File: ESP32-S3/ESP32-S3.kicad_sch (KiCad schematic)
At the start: 4 parts, among them J1 Conn_01x08, J2 FlySky Receiver, J3 Conn_01x08, U1 ESP32-S3-DevKitC-1-N32R16V

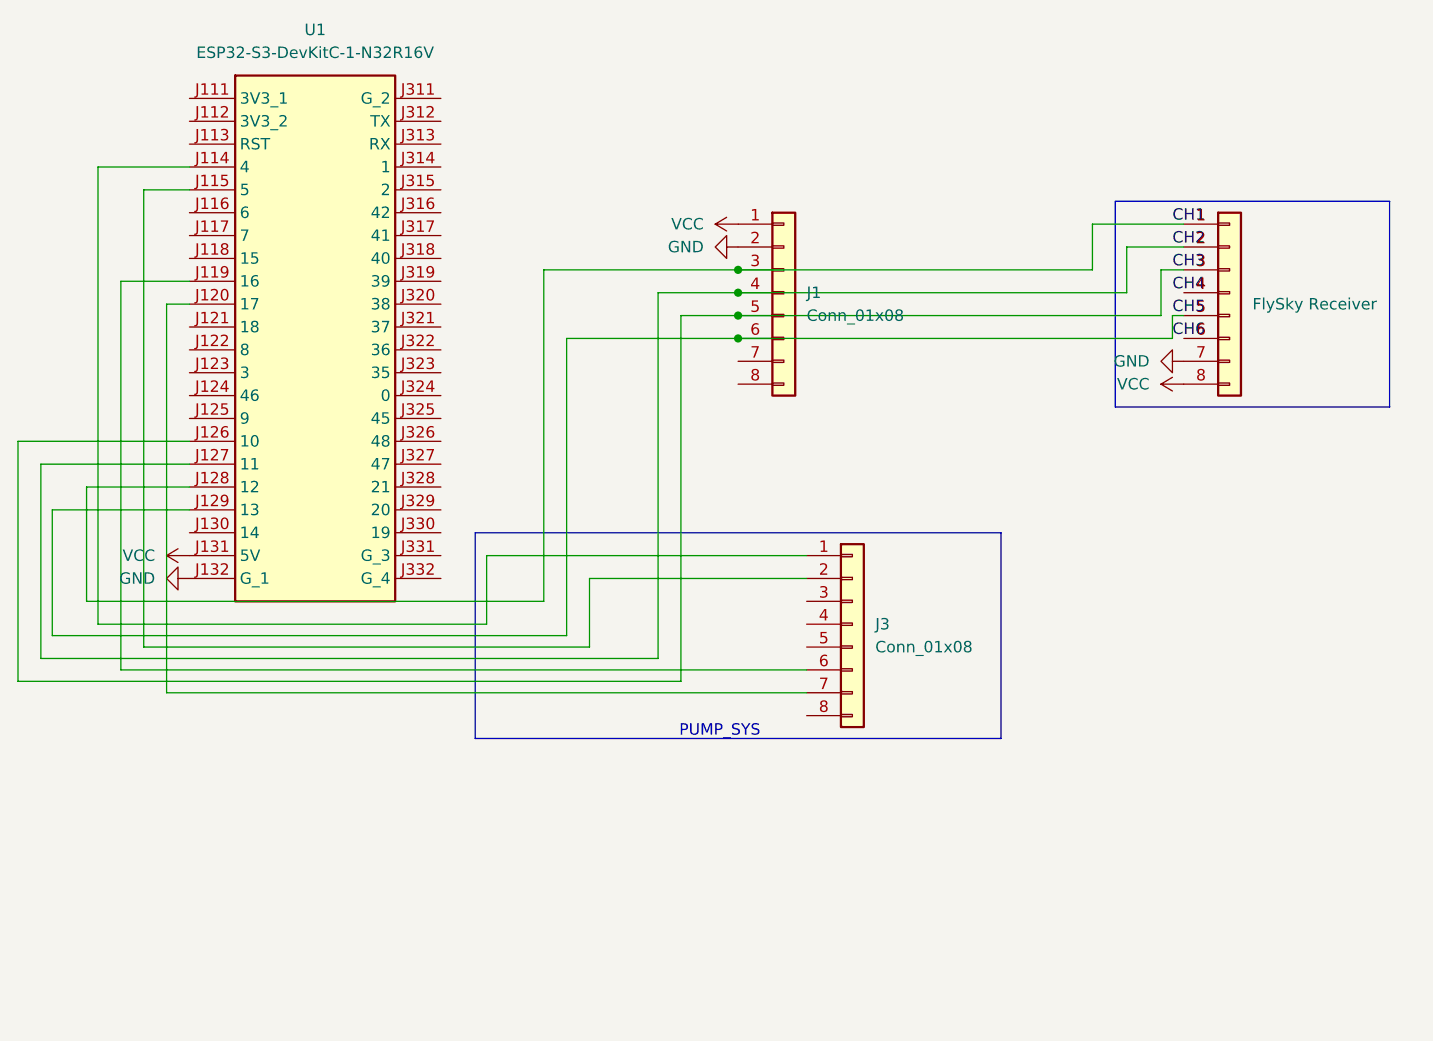
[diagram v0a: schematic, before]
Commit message: Add files via upload
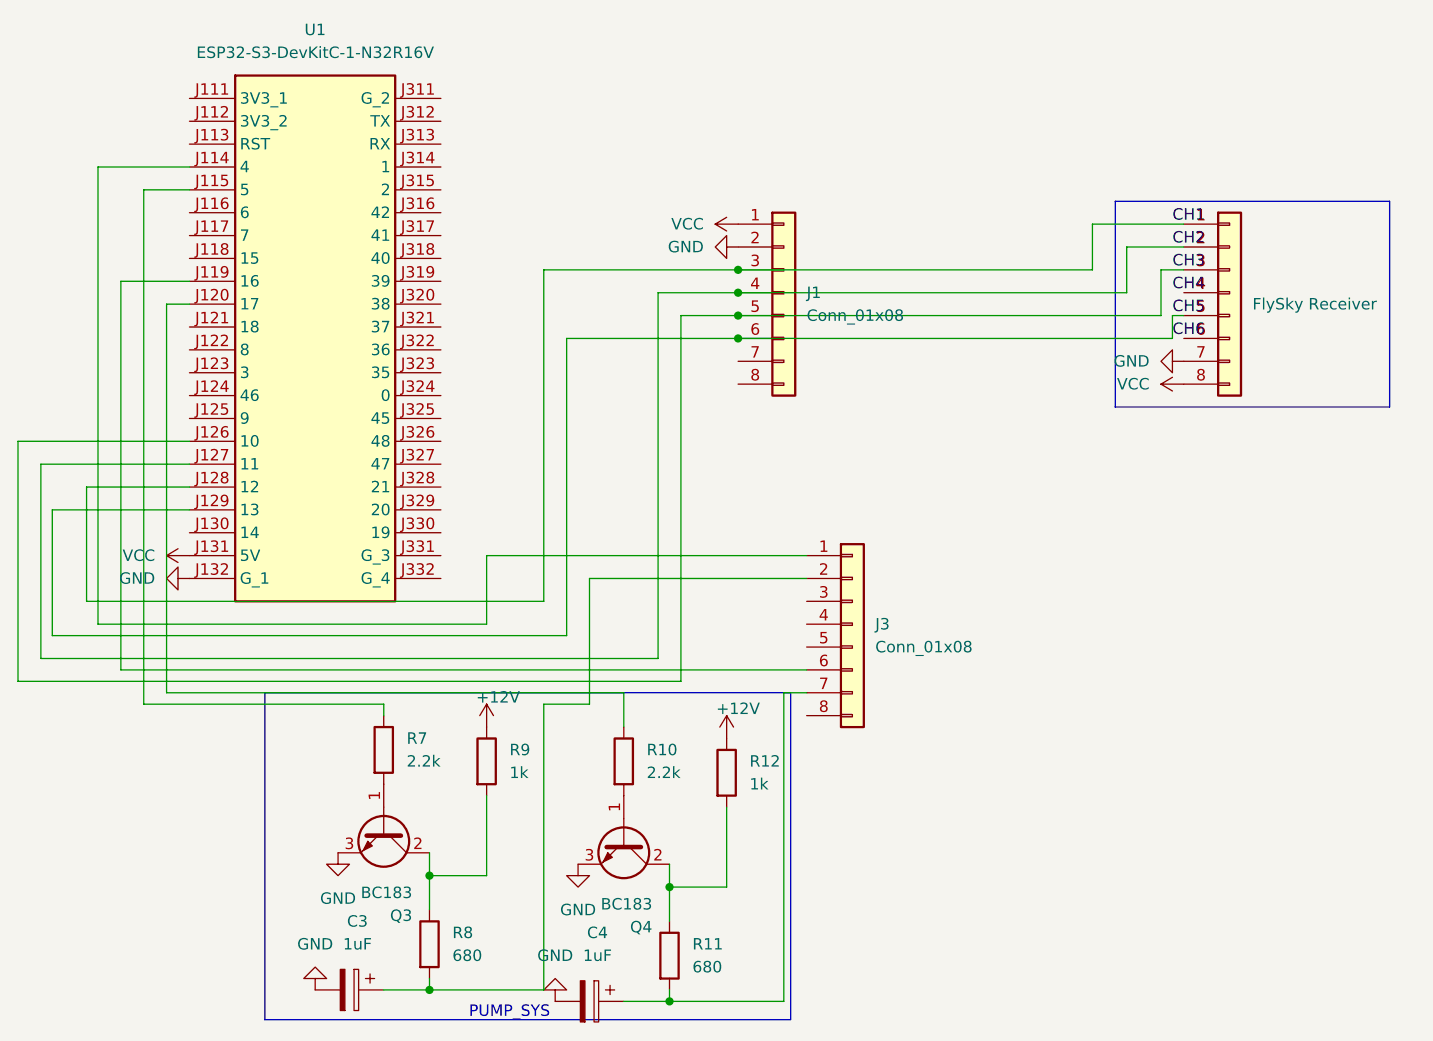
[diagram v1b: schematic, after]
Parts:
- added C3, C4: 1uF, Capacitor_THT:CP_Radial_D5.0mm_P2.00mm, symbol Device:C_Polarized
- added Q3, Q4: BC183, Package_TO_SOT_THT:TO-92_Inline, symbol Transistor_BJT:Q_NPN_BCE
- added R10, R7: 2.2k, Resistor_THT:R_Axial_DIN0207_L6.3mm_D2.5mm_P10.16mm_Horizontal, symbol Device:R
- added R11, R8: 680, Resistor_THT:R_Axial_DIN0207_L6.3mm_D2.5mm_P10.16mm_Horizontal, symbol Device:R
- added R12, R9: 1k, Resistor_THT:R_Axial_DIN0207_L6.3mm_D2.5mm_P10.16mm_Horizontal, symbol Device:R
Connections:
- net GND: now also C3.2, C4.2, Q3.3 (E), Q4.3 (E)
- net at U1.J115 (5): now also R7.1; no longer J3.2 (Pin_2)
- net at U1.J120 (17): now also R10.1; no longer J3.7 (Pin_7)
- new net: Q4.1 (B), R10.2
- new net: Q4.2 (C), R11.1, R12.2
- new net: C4.1, J3.7 (Pin_7), R11.2
- new net: Q3.1 (B), R7.2
- new net: Q3.2 (C), R8.1, R9.2
- new net: C3.1, J3.2 (Pin_2), R8.2
- new net +12V: R12.1, R9.1
